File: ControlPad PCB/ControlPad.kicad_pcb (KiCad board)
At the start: 2 copper layers, 19 parts, among them SW1 SW_Push, SW10 SW_Push, SW2 SW_Push, SW3 SW_Push, SW4 SW_Push, SW6 SW_Push, SW7 SW_Push, SW8 SW_Push, SW9 SW_Push, U1 MOUDLE-SEEEDUINO-XIAO

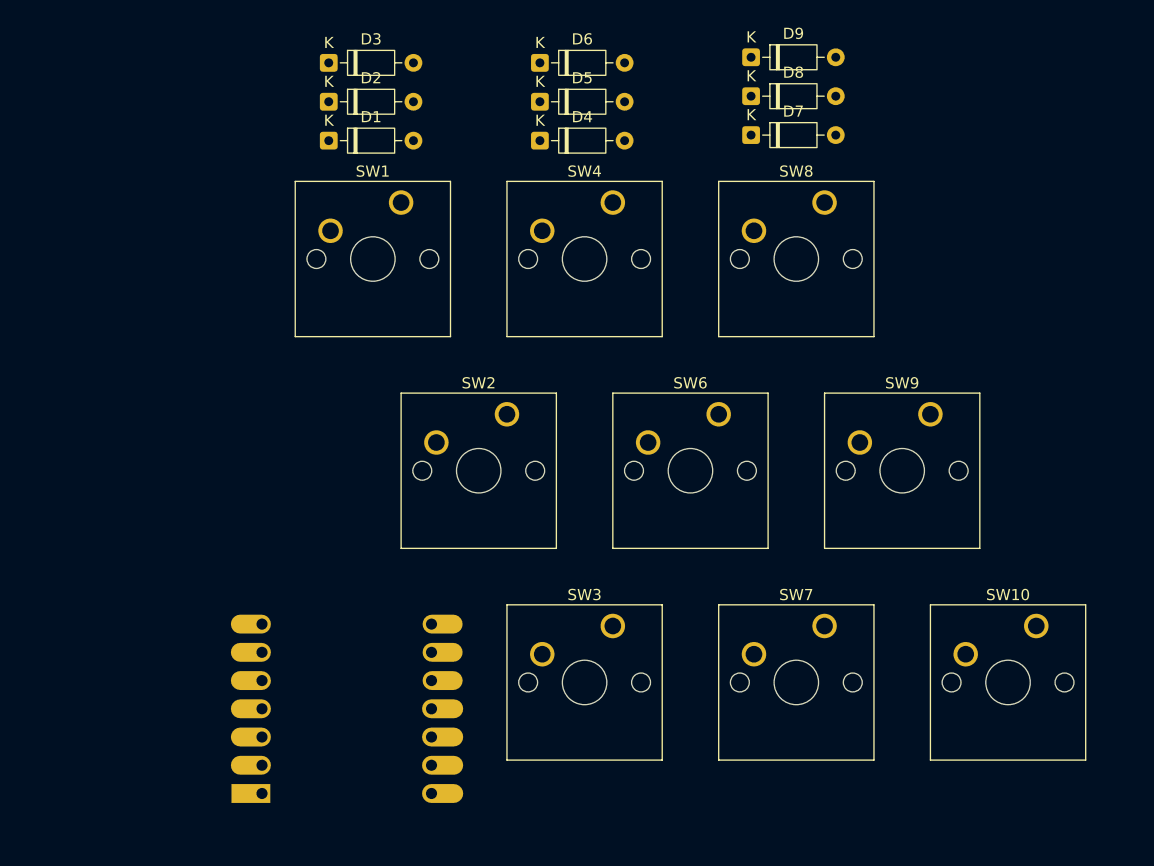
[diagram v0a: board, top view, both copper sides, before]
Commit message: Traces Routing V1
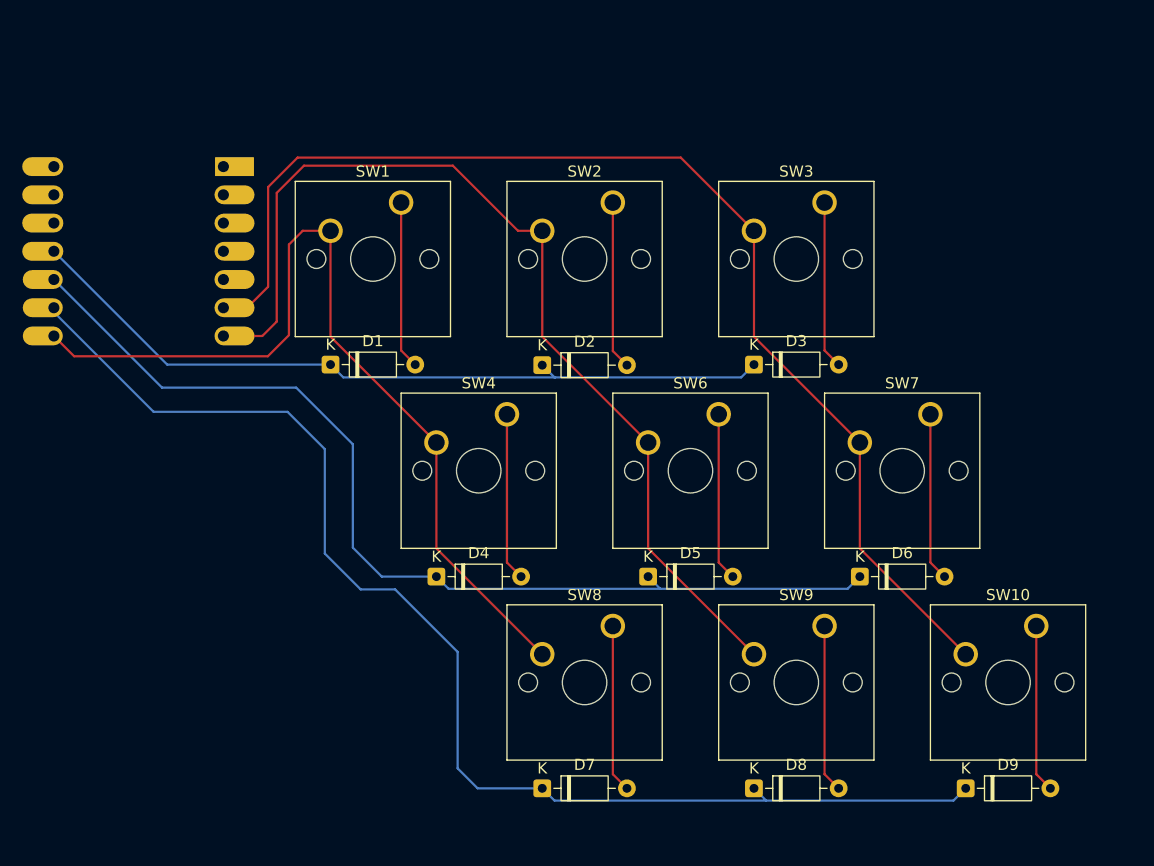
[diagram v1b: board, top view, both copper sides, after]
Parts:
- moved D9 68.6 mm to (186.7, 104.8)
- moved D8 62.3 mm to (167.6, 104.8)
- moved D7 61.7 mm to (148.6, 104.8)
- moved D6 54.5 mm to (177.2, 85.7)
- moved D3 46.9 mm to (167.6, 66.7)
- moved U1 45.2 mm to (112.3, 56.5), turned to 180 degrees
- moved D5 43.8 mm to (158.1, 85.7)
- moved SW3 42.6 mm to (174.0, 52.1)
- moved SW8 42.6 mm to (154.9, 90.2)
- moved D4 40.3 mm to (139.1, 85.7)
- moved D2 30.5 mm to (148.6, 66.7)
- moved SW2 21.3 mm to (154.9, 52.1)
- moved SW4 21.3 mm to (145.4, 71.1)
- moved SW7 21.3 mm to (183.5, 71.1)
- moved SW9 21.3 mm to (174.0, 90.2)
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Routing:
- net Net-(D7-K): track 0.00 -> 114.3 mm
- net Net-(U1-PA9_A5_D5_SCL): track 0.00 -> 107.3 mm
- net Net-(D4-K): track 0.00 -> 91.5 mm
- net Net-(U1-PB08_A6_D6_TX): track 0.00 -> 90.2 mm
- net Net-(U1-PB09_A7_D7_RX): track 0.00 -> 81.1 mm
- net Net-(D1-K): track 0.00 -> 69.8 mm
- net Net-(D2-A): track 0.00 -> 15.2 mm
- net Net-(D9-A): track 0.00 -> 15.1 mm
- net Net-(D7-A): track 0.00 -> 15.1 mm
- net Net-(D6-A): track 0.00 -> 15.1 mm
- net Net-(D5-A): track 0.00 -> 15.1 mm
- net Net-(D4-A): track 0.00 -> 15.1 mm
- net Net-(D8-A): track 0.00 -> 15.1 mm
- net Net-(D1-A): track 0.00 -> 15.1 mm
- net Net-(D3-A): track 0.00 -> 15.1 mm

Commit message: Traces Routing V2
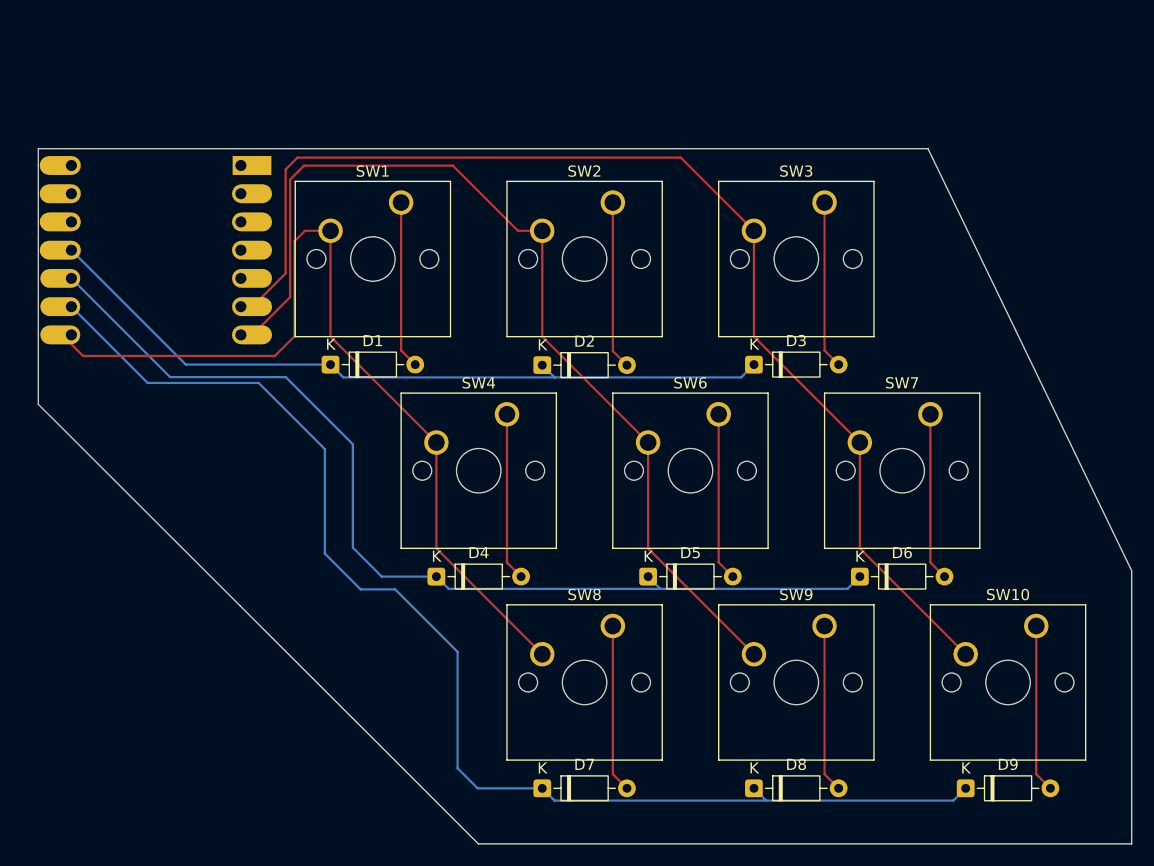
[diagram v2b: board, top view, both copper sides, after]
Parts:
- moved U1 1.58 mm to (113.8, 56.4)
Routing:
- net Net-(U1-PB08_A6_D6_TX): track 90.2 -> 88.0 mm
- net Net-(D4-K): track 91.5 -> 90.0 mm
- net Net-(D1-K): track 69.8 -> 68.2 mm
- net Net-(U1-PA9_A5_D5_SCL): track 107.3 -> 105.9 mm
- net Net-(D7-K): track 114.3 -> 112.9 mm
- net Net-(U1-PB09_A7_D7_RX): track 81.1 -> 80.3 mm
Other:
- board outline added: 98.4 x 62.6 mm
